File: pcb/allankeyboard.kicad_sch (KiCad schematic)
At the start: 161 parts, among them U1 Nice_Nano_V2

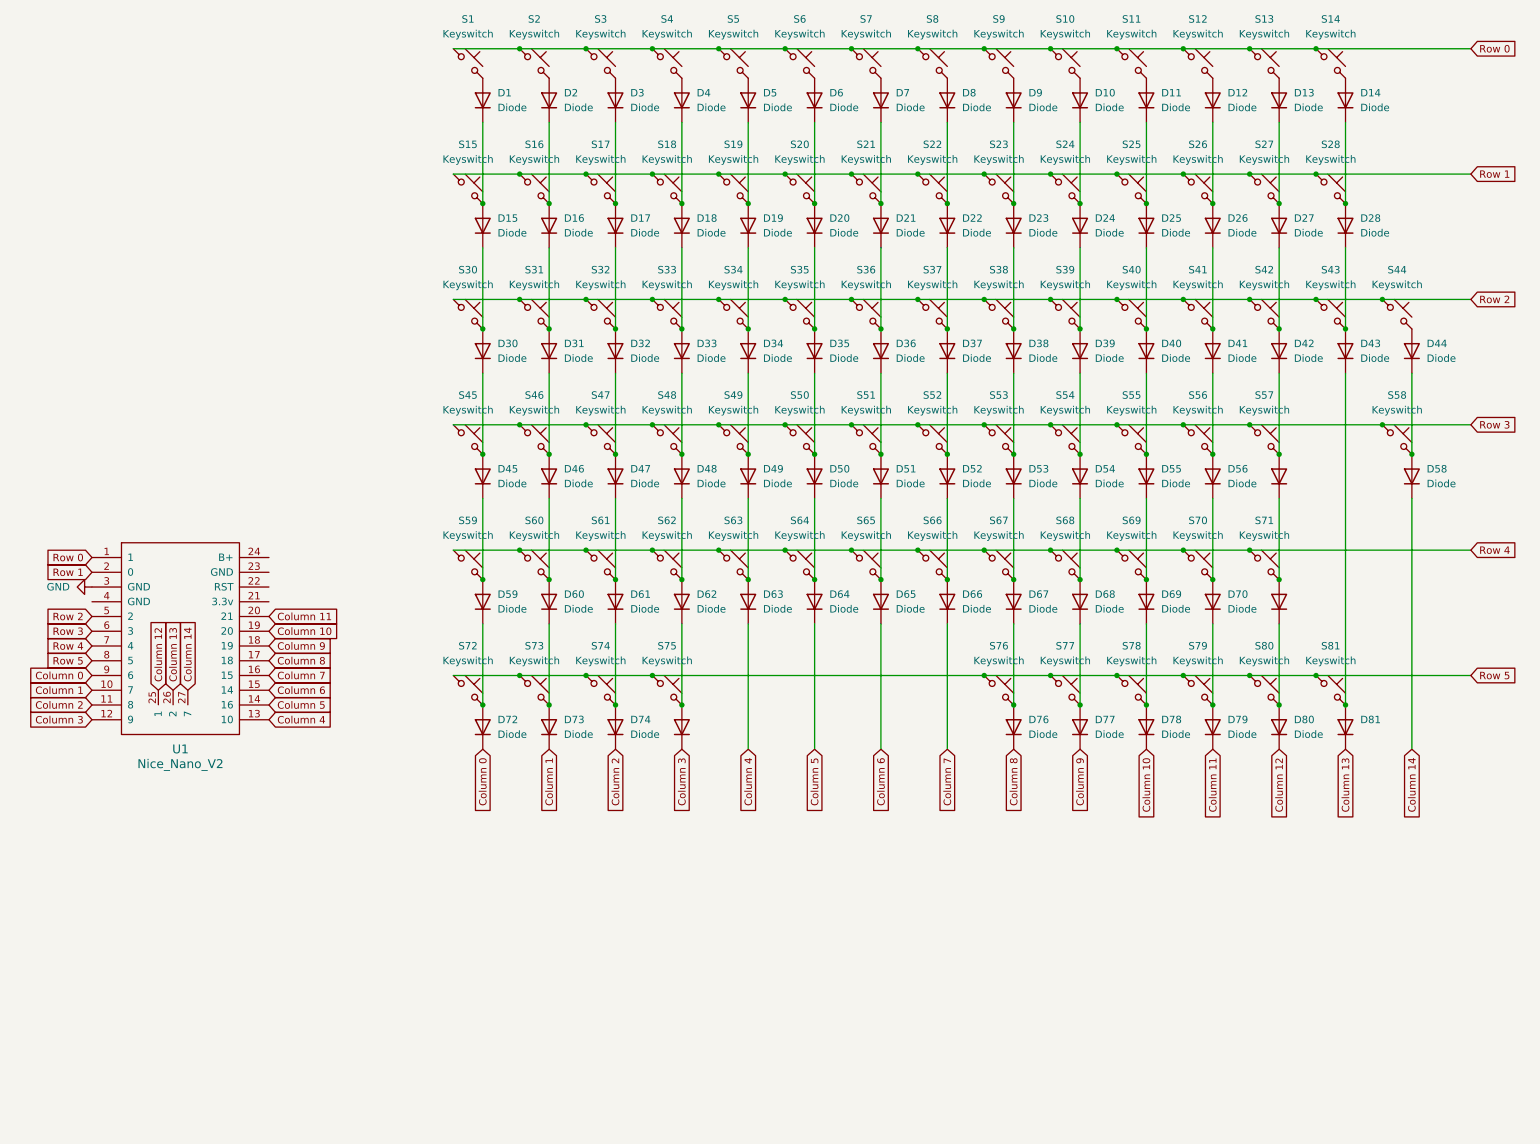
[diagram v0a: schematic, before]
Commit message: Finished Jounraling, added all step files and complete BOM
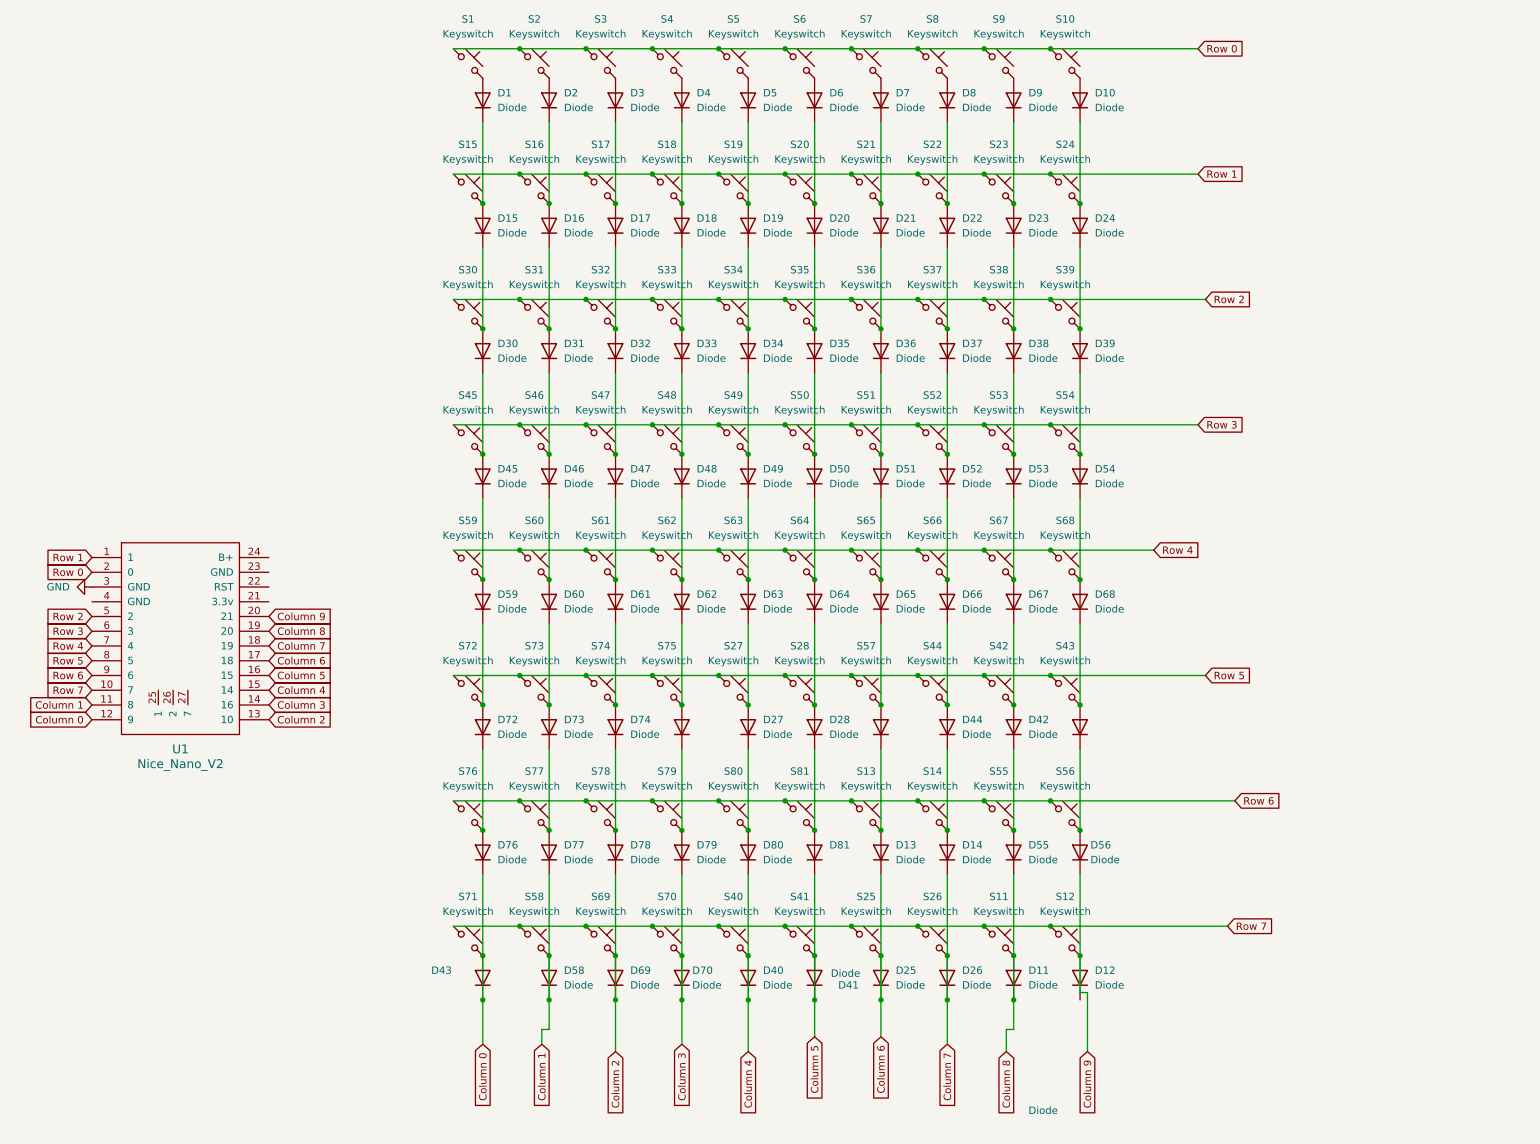
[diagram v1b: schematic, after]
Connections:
- net Column 0: now also D71.1 (K), D71.2 (A), D76.1 (K), S71.2, U1.12 (9); no longer D72.1 (K), U1.9 (6)
- net Column 1: now also D58.1 (K), D58.2 (A), D77.1 (K), S58.2, U1.11 (8); no longer D73.1 (K), U1.10 (7)
- net Column 2: now also D69.1 (K), D69.2 (A), D78.1 (K), S69.2, U1.13 (10); no longer D74.1 (K), U1.11 (8)
- net Column 3: now also D70.1 (K), D70.2 (A), D79.1 (K), S70.2, U1.14 (16); no longer D75.1 (K), U1.12 (9)
- net Column 4: now also D40.1 (K), D40.2 (A), D80.1 (K), S40.2, U1.15 (14); no longer D63.1 (K), U1.13 (10)
- net Column 5: now also D41.1 (K), D41.2 (A), D81.1 (K), S41.2, U1.16 (15); no longer D64.1 (K), U1.14 (16)
- net Column 6: now also D13.1 (K), D25.1 (K), D25.2 (A), S25.2, U1.17 (18); no longer D65.1 (K), U1.15 (14)
- net Column 7: now also D14.1 (K), D26.1 (K), D26.2 (A), S26.2, U1.18 (19); no longer D66.1 (K), U1.16 (15)
- net Column 8: now also D11.1 (K), D11.2 (A), D55.1 (K), S11.2, U1.19 (20); no longer D76.1 (K), U1.17 (18)
- net Column 9: now also D12.2 (A), D56.1 (K), S12.2, U1.20 (21); no longer D77.1 (K), U1.18 (19)
- net Row 0: now also U1.2 (0); no longer S11.1, S12.1, S13.1, S14.1, U1.1
- net Row 1: now also U1.1; no longer S25.1, S26.1, S27.1, S28.1, U1.2 (0)
- net Row 2: no longer S40.1, S41.1, S42.1, S43.1, S44.1
- net Row 3: no longer S55.1, S56.1, S57.1, S58.1
- net Row 4: no longer S69.1, S70.1, S71.1
- net Row 5: now also S27.1, S28.1, S42.1, S43.1, S44.1, S57.1; no longer S76.1, S77.1, S78.1, S79.1, S80.1, S81.1
- net at D13.2 (A), S13.2: now also D57.1 (K)
- net at D57.2 (A), S57.2: now also D65.1 (K); no longer D42.1 (K)
- net at D77.2 (A), S77.2: now also D73.1 (K); no longer D68.1 (K)
- net at D78.2 (A), S78.2: now also D74.1 (K); no longer D69.1 (K)
- net at D80.2 (A), S80.2: now also D27.1 (K); no longer D71.1 (K)
- net at D79.2 (A), S79.2: now also D75.1 (K); no longer D70.1 (K)
- net at D56.2 (A), S56.2: now also D43.1 (K); no longer D41.1 (K)
- net at D76.2 (A), S76.2: now also D72.1 (K); no longer D67.1 (K)
- net at D55.2 (A), S55.2: now also D42.1 (K); no longer D40.1 (K)
- net at D81.2 (A), S81.2: now also D28.1 (K); no longer D43.1 (K)
- net at D43.2 (A), S43.2: now also D68.1 (K); no longer D28.1 (K)
- net at D27.2 (A), S27.2: now also D63.1 (K); no longer D13.1 (K)
- net at D44.2 (A), S44.2: now also D66.1 (K)
- net at D28.2 (A), S28.2: now also D64.1 (K); no longer D14.1 (K)
- net at D42.2 (A), S42.2: now also D67.1 (K); no longer D27.1 (K)
- net at D14.2 (A), S14.2: now also D44.1 (K)
- removed net Column 10: D78.1 (K), U1.19 (20)
- removed net Column 11: D79.1 (K), U1.20 (21)
- net Column 12: no longer names the net of U1.25 (1)
- net Column 12: no longer D80.1 (K)
- net Column 13: no longer names the net of U1.26 (2)
- net Column 13: no longer D81.1 (K)
- net Column 14: no longer names the net of U1.27 (7)
- net Column 14: no longer D58.1 (K)
- new net Row 6: S13.1, S14.1, S55.1, S56.1, S76.1, S77.1, S78.1, S79.1, S80.1, S81.1, U1.9 (6)
- new net Row 7: S11.1, S12.1, S25.1, S26.1, S40.1, S41.1, S58.1, S69.1, S70.1, S71.1, U1.10 (7)
- now unconnected: D12.1 (K)
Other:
- moved on the sheet: D11, D12, D13, D14, D25, D26, D27, D28, D40, D41, D42, D43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
